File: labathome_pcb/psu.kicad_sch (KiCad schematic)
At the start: 21 parts, among them J8 POWER, SW11 PROG 5V POWER, U11 FUSB302BMPX, U24 SRV05, U9 RY8310

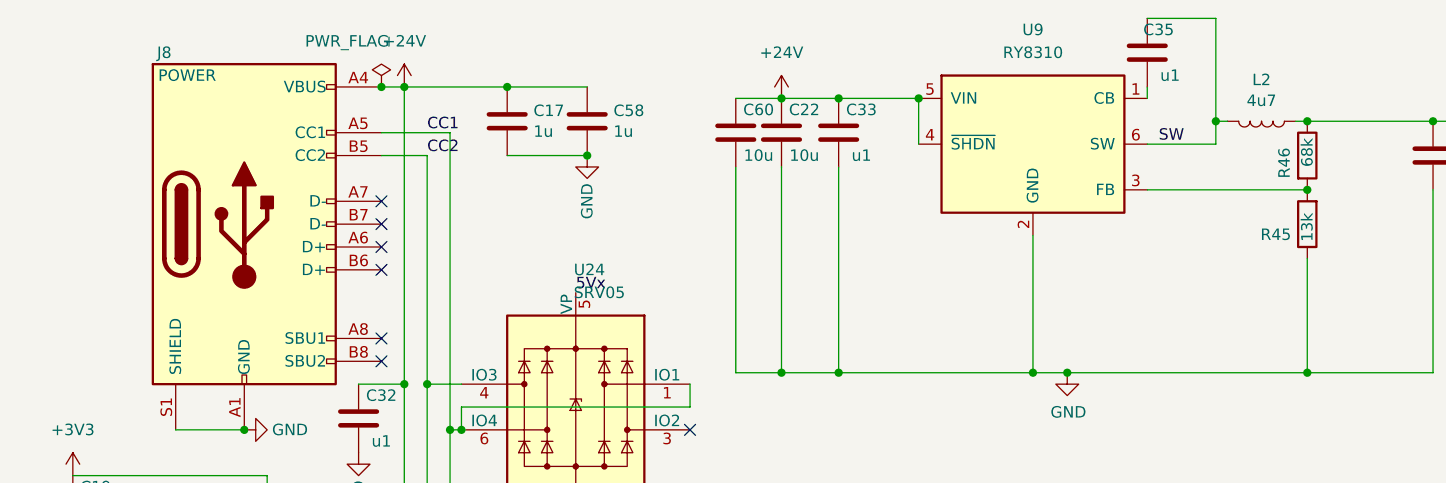
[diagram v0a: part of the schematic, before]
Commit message: Modbus Firmware
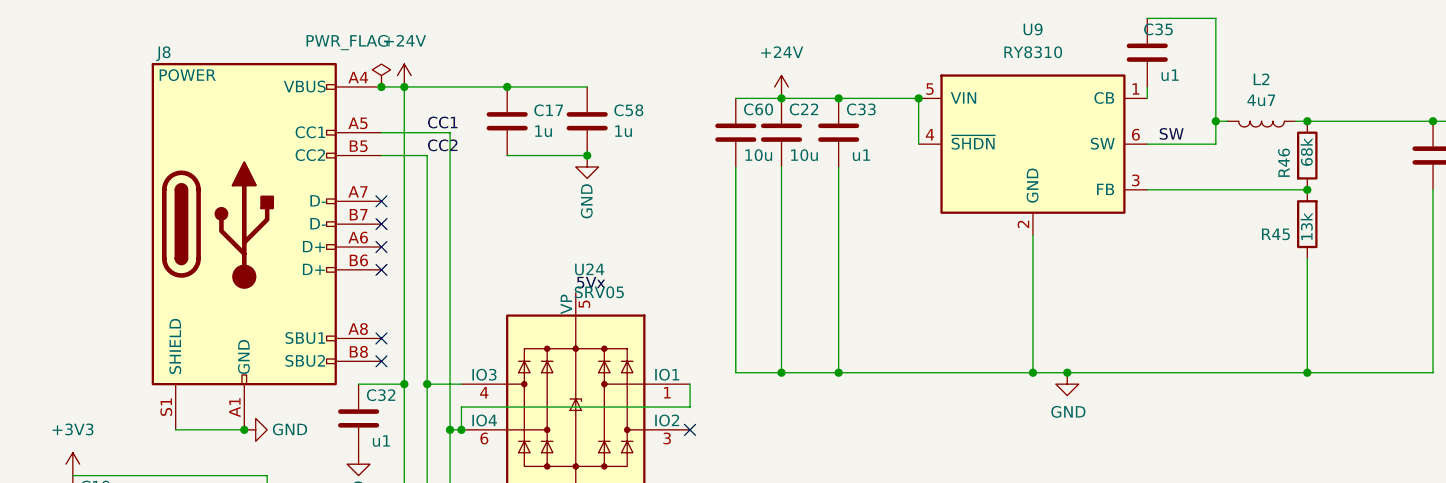
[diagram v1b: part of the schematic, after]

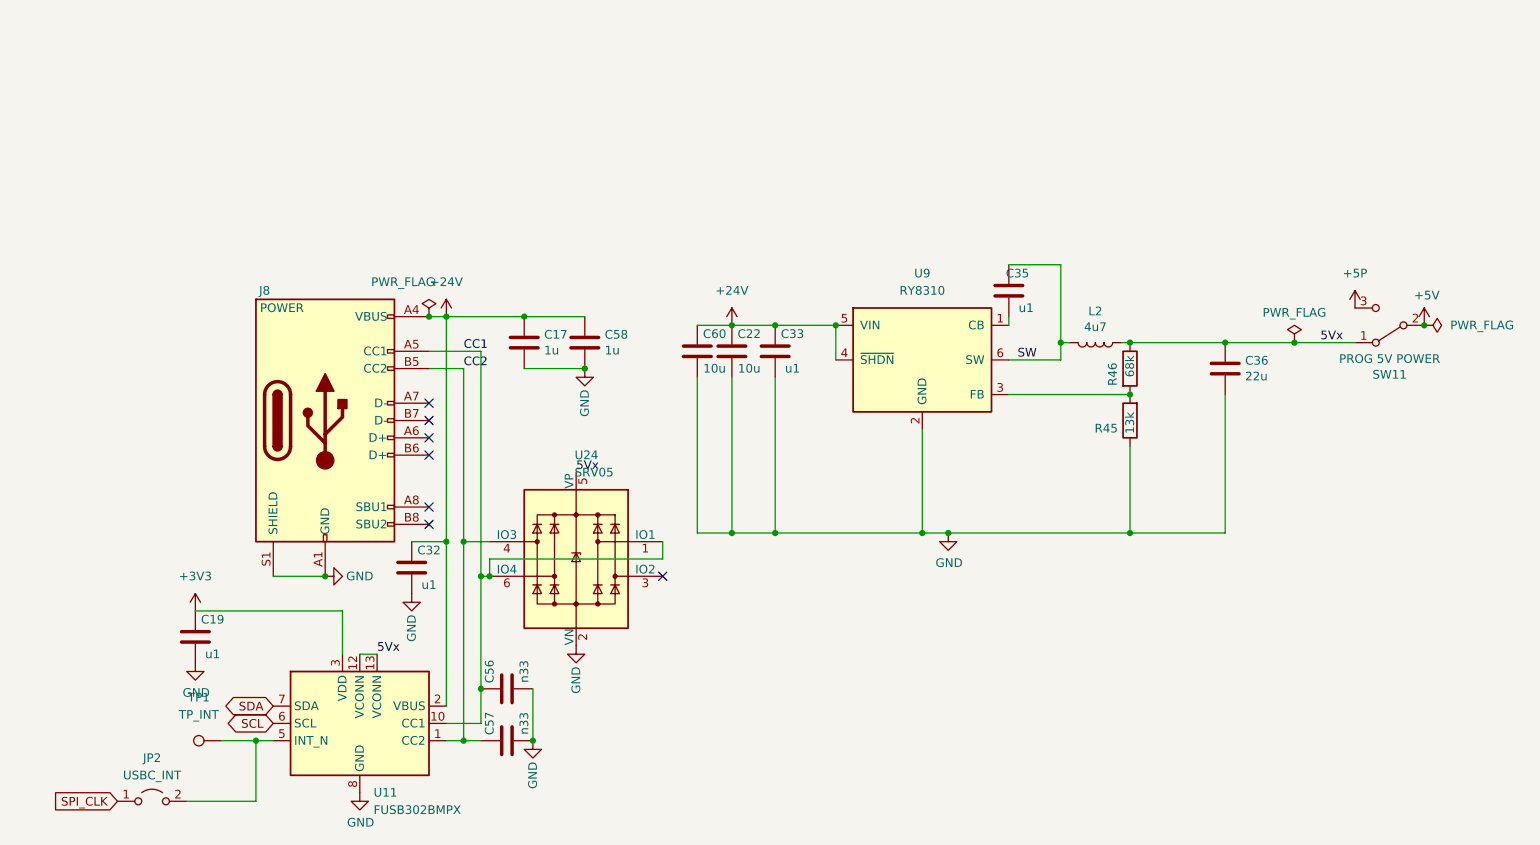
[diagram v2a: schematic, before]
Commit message: Reorganization of code
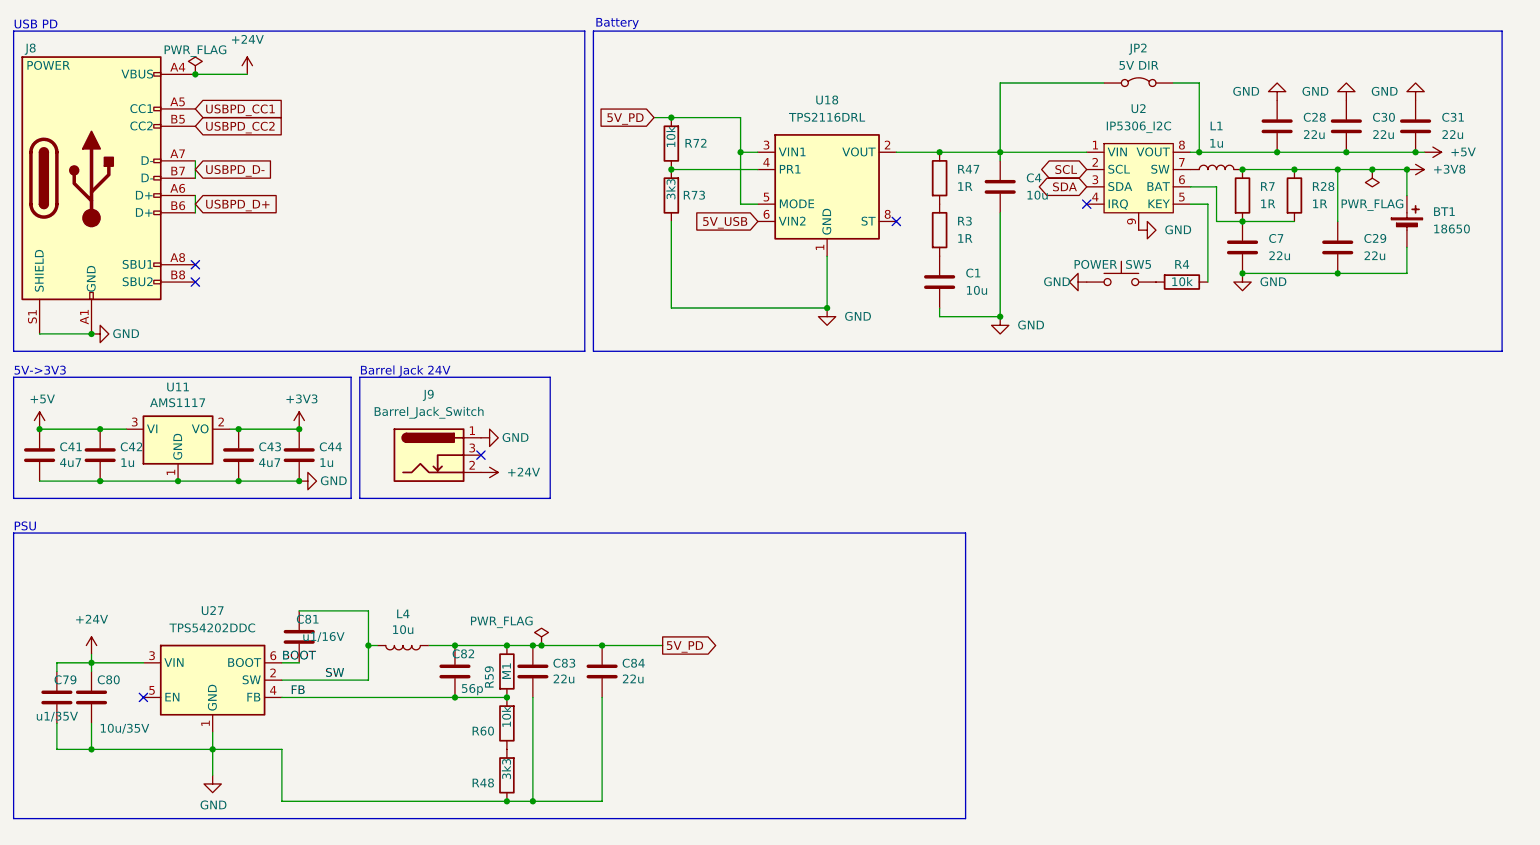
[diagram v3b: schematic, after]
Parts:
- removed C17, C58: 1u, Capacitor_SMD:C_1206_3216Metric, symbol Device:C
- removed C19, C32, C33, C35: u1, Capacitor_SMD:C_0603_1608Metric, symbol Device:C
- removed C22, C60: 10u, Capacitor_SMD:C_1206_3216Metric, symbol Device:C
- removed C36: 22u, Capacitor_SMD:C_0603_1608Metric, symbol Device:C
- removed C56, C57: n33, Capacitor_SMD:C_0603_1608Metric, symbol Device:C
- removed J8: POWER, liebler_CONN:USB_C_Receptacle_HRO_TYPE-C-31-M-12_IMPROVED, symbol Connector:USB_C_Receptacle_USB2.0
- removed JP2: USBC_INT, liebler_CONN:Jumper_Trace_025x150x015, symbol Jumper:Jumper_2_Open
- removed L2: 4u7, Inductor_SMD:L_Abracon_ASPI-0630LR, symbol Device:L
- removed R45: 13k, Resistor_SMD:R_0603_1608Metric, symbol Device:R
- removed R46: 68k, Resistor_SMD:R_0603_1608Metric, symbol Device:R
- removed SW11: PROG 5V POWER, liebler_MECH:Switch_SS12D00, symbol Switch:SW_SPDT
- removed TP1: TP_INT, TestPoint:TestPoint_THTPad_1.0x1.0mm_Drill0.5mm, symbol Connector:TestPoint
- removed U11: FUSB302BMPX, Package_DFN_QFN:WQFN-14-1EP_2.5x2.5mm_P0.5mm_EP1.45x1.45mm, symbol Interface_USB:FUSB302BMPX
- removed U24: SRV05, Package_TO_SOT_SMD:SOT-23-6, symbol Power_Protection:SRV05-4
- removed U9: RY8310, Package_TO_SOT_SMD:SOT-23-6, symbol Regulator_Switching:LMR14206
- added BT1: 18650, Battery:BatteryHolder_MPD_BH-18650-PC2, symbol Device:Battery_Cell
- added C1, C4: 10u, Capacitor_SMD:C_0805_2012Metric, symbol Device:C
- added C28, C29, C30, C31, C7, C83, C84: 22u, Capacitor_SMD:C_0603_1608Metric, symbol Device:C
- added C41, C43: 4u7, Capacitor_SMD:C_0402_1005Metric, symbol Device:C
- added C42, C44: 1u, Capacitor_SMD:C_0402_1005Metric, symbol Device:C
- added C79: u1/35V, Capacitor_SMD:C_0603_1608Metric, symbol Device:C
- added C80: 10u/35V, Capacitor_SMD:C_0805_2012Metric, symbol Device:C
- added C81: u1/16V, Capacitor_SMD:C_0603_1608Metric, symbol Device:C
- added C82: 56p, Capacitor_SMD:C_0402_1005Metric, symbol Device:C
- added J8: POWER, liebler_CONN:USB_C_Receptacle_HRO_TYPE-C-31-M-12_IMPROVED, symbol Connector:USB_C_Receptacle_USB2.0_16P
- added J9: Barrel_Jack_Switch, Connector_BarrelJack:BarrelJack_Horizontal, symbol Connector:Barrel_Jack_Switch
- added JP2: 5V DIR, Jumper:SolderJumper-2_P1.3mm_Bridged2Bar_Pad1.0x1.5mm, symbol Jumper:Jumper_2_Bridged
- added L1: 1u, liebler_PASSIVES:L_0630, symbol Device:L
- added L4: 10u, liebler_PASSIVES:L_0630, symbol Device:L
- added R28, R3, R47, R7: 1R, Resistor_SMD:R_0603_1608Metric, symbol Device:R
- added R4, R60, R72: 10k, Resistor_SMD:R_0201_0603Metric, symbol Device:R
- added R48, R73: 3k3, Resistor_SMD:R_0402_1005Metric, symbol Device:R
- added R59: M1, Resistor_SMD:R_0201_0603Metric, symbol Device:R
- added SW5: POWER, liebler_MECH:SW_Push_1P1T_NO_6x6mm_H6.5mm_Reverse, symbol Switch:SW_Push
- added U11: AMS1117, Package_TO_SOT_SMD:SOT-223-3_TabPin2, symbol Regulator_Linear:AMS1117-3.3
- added U18: TPS2116DRL, Package_TO_SOT_SMD:SOT-583-8, symbol Power_Management:TPS2116DRL
- added U2: IP5306_I2C, Package_SO:HSOP-8-1EP_3.9x4.9mm_P1.27mm_EP2.3x2.3mm_ThermalVias, symbol liebler_SEMICONDUCTORS:IP5306_I2C
- added U27: TPS54202DDC, Package_TO_SOT_SMD:SOT-23-6_Handsoldering, symbol Regulator_Switching:TPS54202DDC
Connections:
- net +24V: now also C79.2, C80.2, J8.A4 (VBUS), J8.A9 (VBUS), J8.B4 (VBUS), J8.B9 (VBUS), J9.2, U27.3 (VIN)
- net +3V3: now also C43.2, C44.1, U11.2 (VO)
- net +5V: now also C28.2, C30.2, C31.2, C41.2, C42.1, JP2.2 (B), U11.3 (VI), U2.8 (VOUT)
- net GND: now also BT1.2 (-), C1.2, C28.1, C29.2, C30.1, C31.1, C4.2, C41.1, C42.2, C43.1, C44.2, C7.2, C79.1, C80.1, C83.2, C84.2, J8.A1 (GND), J8.A12 (GND), J8.B1 (GND), J8.B12 (GND), J8.S1 (SHIELD), J9.1, R48.1, R73.1, SW5.1, U11.1 (GND), U18.1 (GND), U2.9, U27.1 (GND)
- net SCL: now also U2.2 (SCL)
- net SDA: now also U2.3 (SDA)
- net SW: now also C81.2, L4.2, U27.2 (SW)
- new net: C4.1, JP2.1 (A), R47.1, U18.2 (VOUT), U18.7 (VOUT), U2.1 (VIN)
- new net: R4.1, U2.5 (KEY)
- new net: C7.1, R28.2, R7.2, U2.6 (BAT)
- new net: L1.1, U2.7 (SW)
- new net: R48.2, R60.1
- new net: R3.1, R47.2
- new net: C1.1, R3.2
- new net: R4.2, SW5.2
- new net: R72.1, R73.2, U18.4 (PR1)
- new net +3V8: BT1.1 (+), C29.1, L1.2, R28.1, R7.1
- new net 5V_PD: C82.2, C83.1, C84.1, L4.1, R59.1, R72.2, U18.3 (VIN1), U18.5 (MODE)
- new net 5V_USB: U18.6 (VIN2)
- new net BOOT: C81.1, U27.6 (BOOT)
- new net FB: C82.1, R59.2, R60.2, U27.4 (FB)
- new net USBPD_CC1: J8.A5 (CC1)
- new net USBPD_CC2: J8.B5 (CC2)
- new net USBPD_D+: J8.A6 (D+), J8.B6 (D+)
- new net USBPD_D-: J8.A7 (D-), J8.B7 (D-)
- no-connect marks 7 -> 6
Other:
- note added: "5V->3V3"
- note added: "Barrel Jack 24V"
- note added: "Battery"
- note added: "PSU"
- note added: "USB PD"
- company: (none) -> Klaus Liebler
- title: (none) -> lab@home
